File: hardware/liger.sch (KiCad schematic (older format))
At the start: 19 parts, among them U1? SPX3819

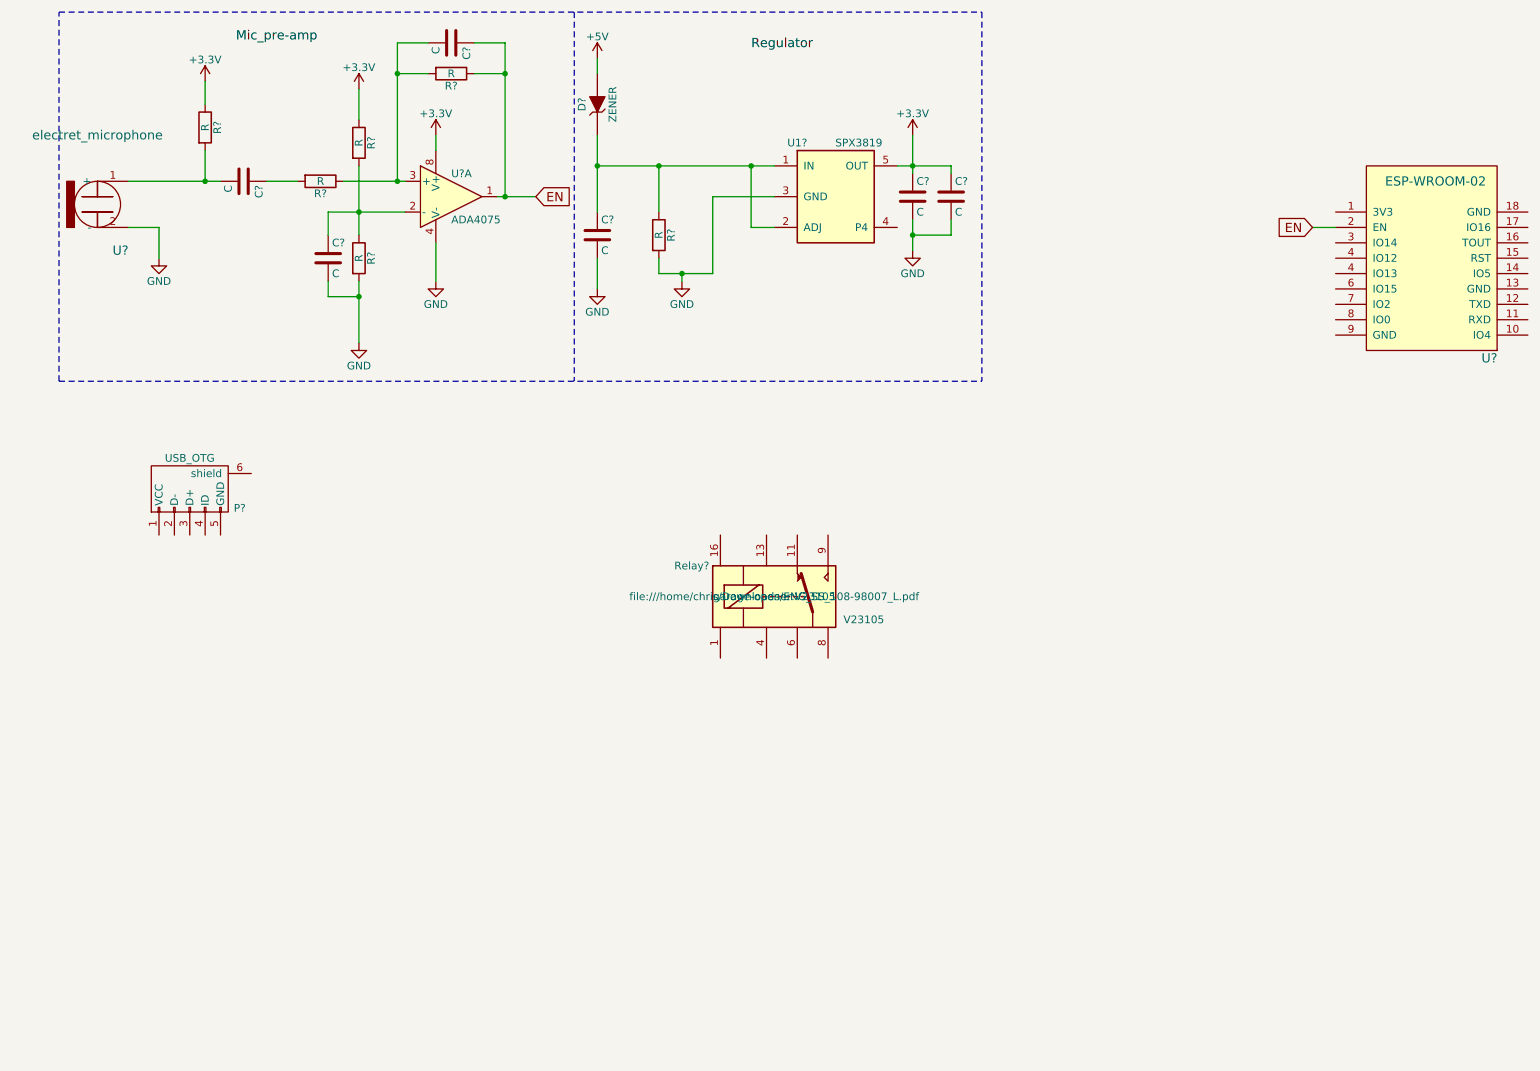
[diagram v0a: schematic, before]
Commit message: liger .2
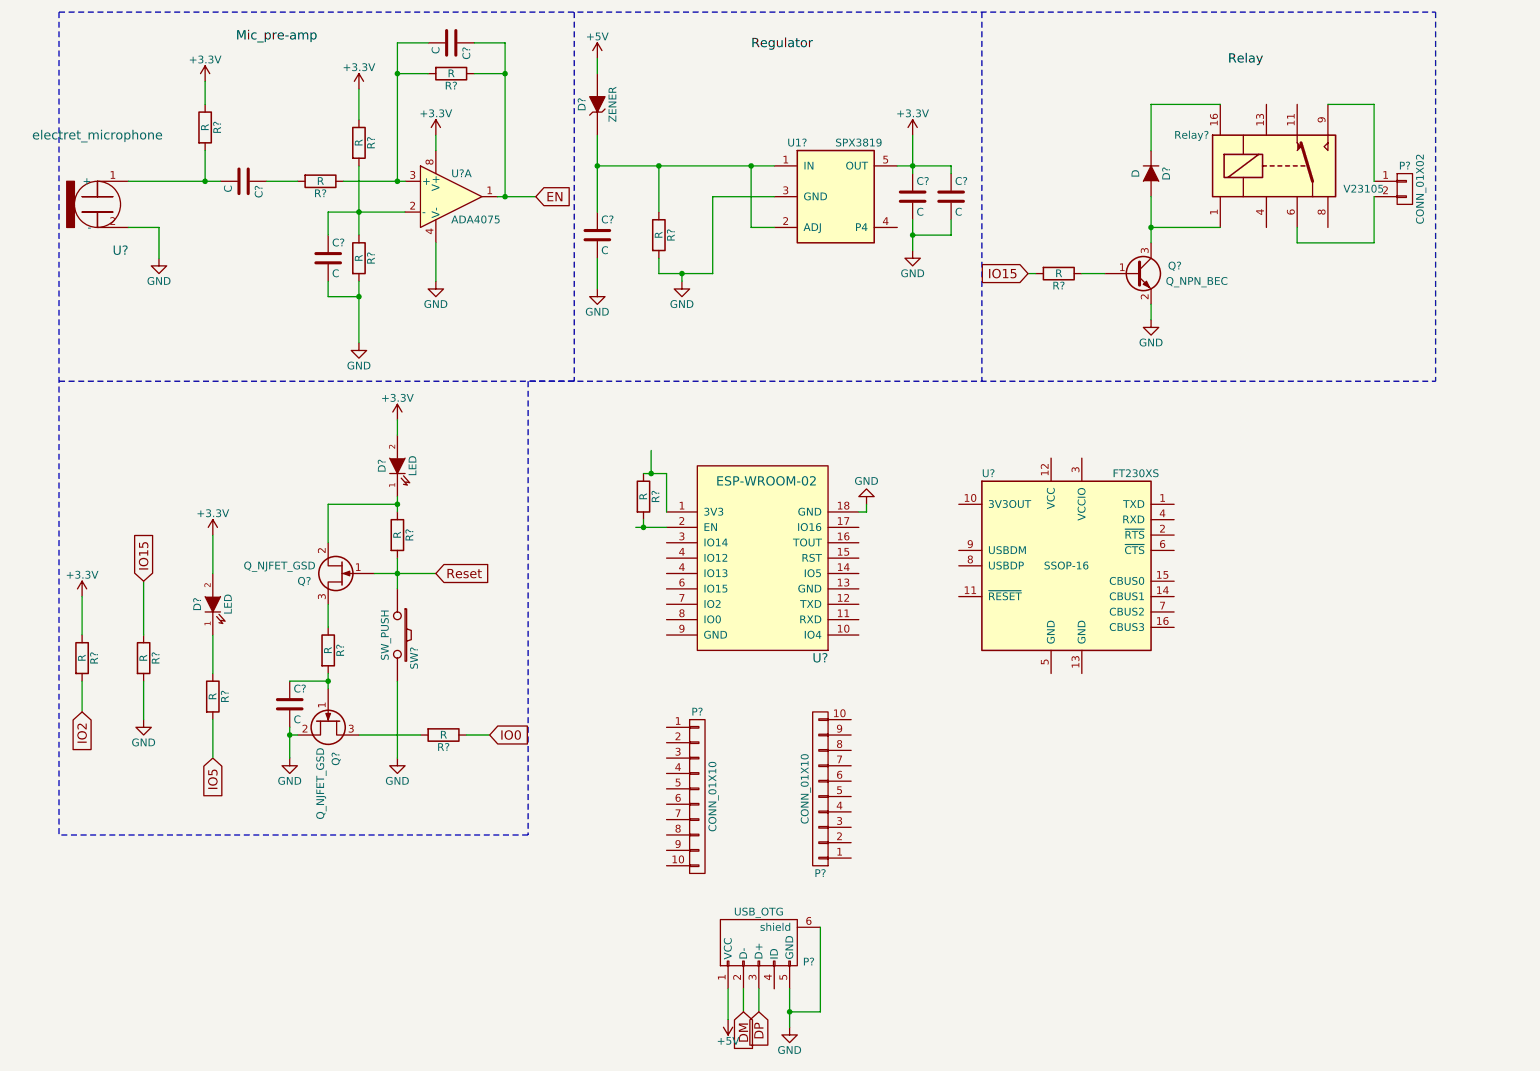
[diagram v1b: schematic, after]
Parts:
- added C?: C, symbol C
- added D?: D, symbol D
- added D? (x2): LED, symbol LED
- added P?: CONN_01X02, symbol CONN_01X02
- added P? (x2): CONN_01X10, symbol CONN_01X10
- added Q?: Q_NPN_BEC, symbol Q_NPN_BEC
- added Q? (x2): Q_NJFET_GSD, symbol Q_NJFET_GSD
- added R? (x8): R, symbol R
- added SW?: SW_PUSH, symbol SW_PUSH
- added U?: FT230XS, SSOP-16, symbol FT230XS
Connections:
- net +3V3: now also D?.2 (A), D?.2 (A), R?.1
- net +5V: now also P?.1 (VCC)
- net EN: no longer U?.2 (EN)
- net GND: now also P?.5 (GND), P?.6 (shield), U?.18 (GND), C?.2, Q?.2 (E), Q?.2 (S), R?.2, SW?.2
- net at Relay?.1: now also D?.2 (A), Q?.3 (C)
- net at Relay?.16: now also D?.1 (K)
- net at Relay?.6: now also P?.2 (P2)
- net at Relay?.9: now also P?.1 (P1)
- net DM: now reaches P?.2 (D-)
- net DP: now reaches P?.3 (D+)
- net at U?.1 (3V3): now also R?.1
- new net: R?.2, U?.2 (EN)
- new net: Q?.1 (B), R?.1
- new net: D?.1 (K), R?.1
- new net: D?.1 (K), Q?.2 (S), R?.1
- new net: Q?.3 (D), R?.2
- new net: Q?.3 (D), R?.1
- new net: C?.1, Q?.1 (G), R?.2
- new net IO0: R?.1
- new net IO15: R?.1, R?.2
- new net IO2: R?.2
- new net IO5: R?.2
- new net Reset: Q?.1 (G), R?.2, SW?.1
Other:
- moved on the sheet: P?, Relay?, U?
